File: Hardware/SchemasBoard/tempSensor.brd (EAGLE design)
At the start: 19.4 x 19 mm, 14 parts, among them IC1 DS1820, T1 BC846

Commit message: a
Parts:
- C1: value (none) -> 100nF
- C2: value (none) -> 1uF
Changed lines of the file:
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@@
 <element name="LSP1" library="solpad" package="LSP11" value="LSP11" x="2.54" y="1.3716"/>
 <element name="LSP2" library="solpad" package="LSP11" value="LSP11" x="15.1384" y="1.3208"/>
-<element name="C1" library="resistor" package="C2012" value="" x="12.5603" y="16.3703" rot="MR90"/>
+<element name="C1" library="resistor" package="C2012" value="100nF" x="12.5603" y="16.3703" rot="MR90"/>
 <element name="S1" library="switch-dil" package="SD4-01" value="" x="5.7658" y="5.9436" rot="R90">
 <attribute name="OC_NEWARK" value="unknown" x="5.7658" y="5.9436" size="1.778" layer="27" rot="R90" display="off"/>
@@
 <attribute name="OC_FARNELL" value="unknown" x="5.7658" y="5.9436" size="1.778" layer="27" rot="R90" display="off"/>
 </element>
-<element name="C2" library="resistor" package="SMC_A" value="" x="14.4145" y="15.9893" rot="MR90"/>
+<element name="C2" library="resistor" package="SMC_A" value="1uF" x="14.4145" y="15.9893" rot="MR90"/>
 <element name="R1" library="resistor" package="R1206W" value="4K7" x="1.524" y="14.9098" rot="MR90"/>
 <element name="JP1" library="pinhead" package="1X03" value="" x="15.2781" y="4.5212"/>

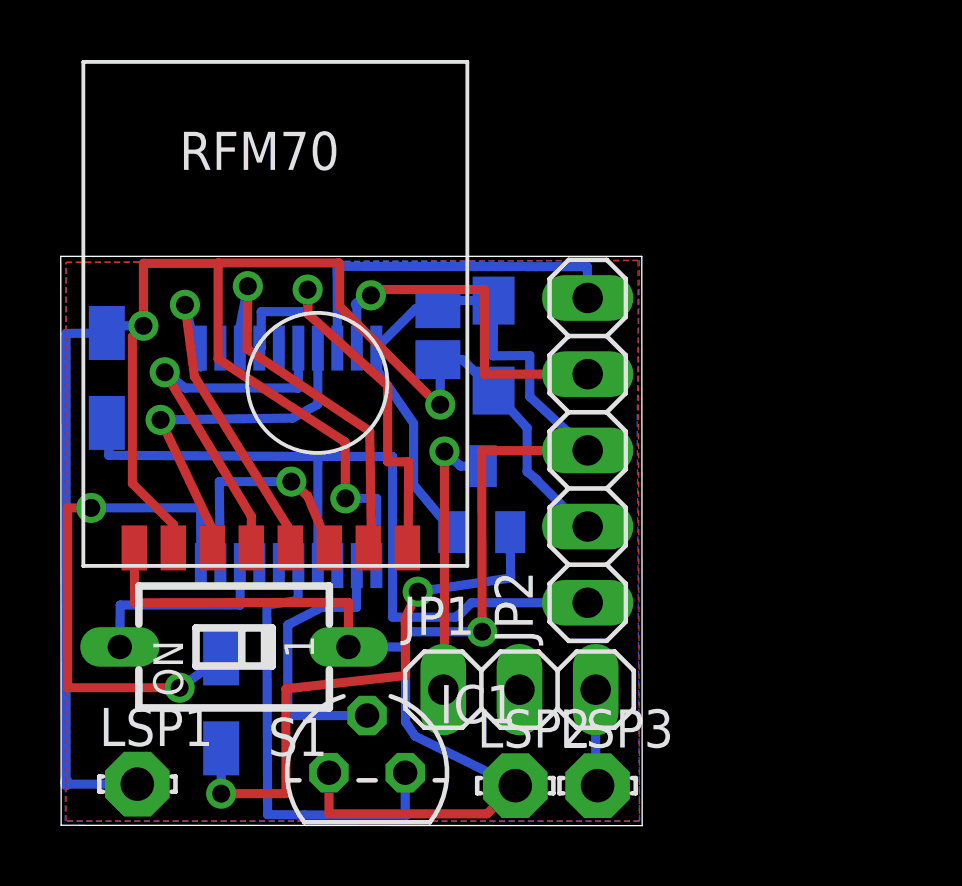
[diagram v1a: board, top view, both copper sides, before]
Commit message: aaa
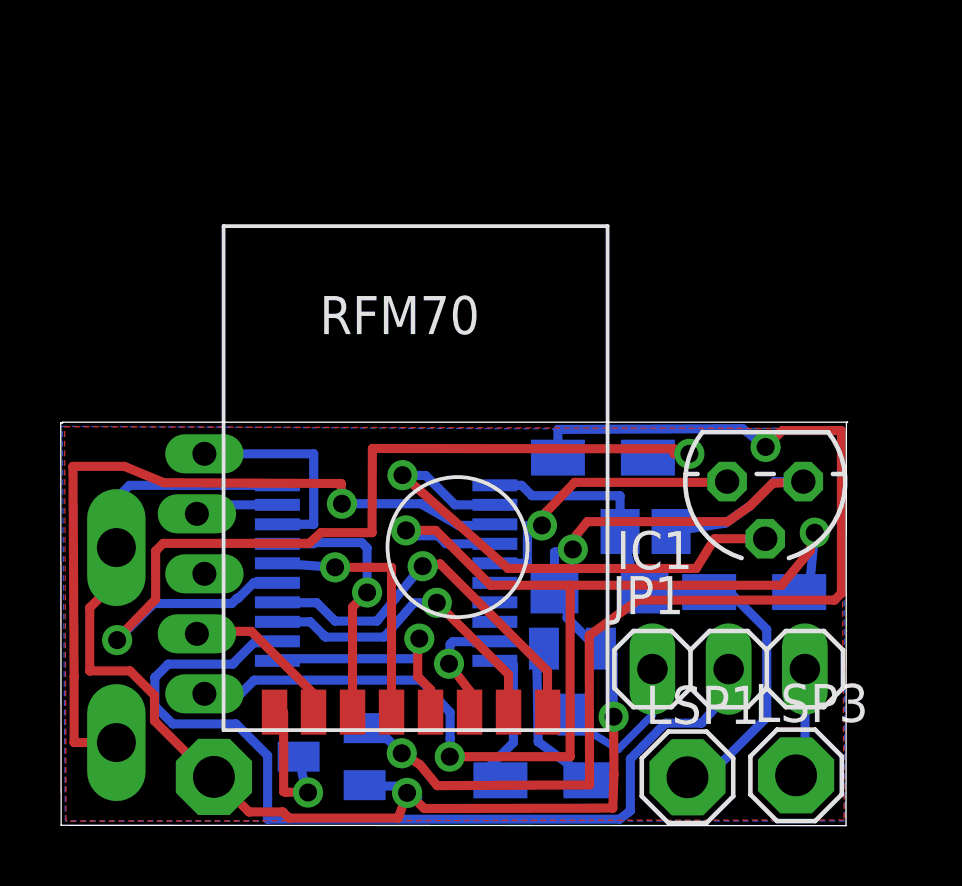
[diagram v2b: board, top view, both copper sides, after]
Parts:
- removed JP2: Prog, pinhead:1X05
- added R3: 1K, resistor:R1206W
- added T2: BC846, transistor:SOT23
- added U$3: PROGRAMMINGHEADERDIP, rfm70:PROGHEADER
- LSP1, LSP2, LSP3: value LSP11 -> SE14; device solpad:LSP11 -> solpad:SE14
- S1: value (none) -> DTS-3; device switch-dil:SD4-01 -> switch-tact:DTS-3
- moved R1 22.7 mm to (23.1, 7.77), turned to 0 degrees
- moved LSP1 18.3 mm to (20.9, 1.60)
- moved IC1 16.4 mm to (23.5, 11.5), turned to 180 degrees
- moved R2 11.1 mm to (16.1, 1.50), turned to 0 degrees
- moved LSP2 10.0 mm to (5.09, 1.61), flipped to the bottom
- moved C1 9.55 mm to (19.5, 9.79), turned to 180 degrees
- moved C2 8.95 mm to (17.9, 7.76), turned to 0 degrees
- moved U$1 7.20 mm to (7.21, 18.1)
- moved JP1 7.01 mm to (22.3, 5.21)
- moved T1 6.79 mm to (17.0, 4.79), turned to 180 degrees
- moved LSP3 6.63 mm to (24.5, 1.66)
- moved U$2 5.06 mm to (10.8, 8.41), turned to 270 degrees
- moved S1 3.92 mm to (1.84, 6.01), flipped to the bottom, turned to 270 degrees
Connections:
- removed net N$18: JP2.4, U$2.19
- removed net N$19: JP2.5, U$2.18
- new net N$10: U$3.GND
- new net N$11: U$2.18, U$3.PGC
- new net N$13: T2.3, U$1.GND
- new net N$14: R3.2, T2.1
- new net N$15: R3.1, U$2.15
- new net N$8: U$2.19, U$3.PGD
- net GND: now also T2.2; no longer JP2.3, U$1.GND
- net N$2: now also U$2.3; no longer U$2.8
- net N$25: now also U$3.MCLR; no longer JP2.1
- net N$4: now also JP1.2
- net VDD: now also U$3.VDD; no longer JP2.2
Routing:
- net VDD: track 66.1 -> 24.1 mm, vias 3 -> 0
- net N$14: track 0.00 -> 38.4 mm, vias 0 -> 2
- net N$15: track 0.00 -> 32.1 mm, vias 0 -> 2
- net N$4: track 0.00 -> 31.0 mm
- net N$2: track 6.71 -> 25.7 mm, vias 0 -> 1
- net N$25: track 26.3 -> 40.8 mm, vias 0 -> 3
- net N$7: track 18.7 -> 5.51 mm, vias 2 -> 0
- net N$6: track 17.8 -> 4.98 mm, vias 2 -> 0
- net N$18: track 12.3 -> 0.00 mm, vias 1 -> 0
- net N$19: track 12.1 -> 0.00 mm
- net N$1: track 9.47 -> 17.3 mm, vias 0 -> 1
- net N$11: track 0.00 -> 7.21 mm
- net N$3: track 15.3 -> 9.75 mm, vias 0 -> 1
- net N$13: track 0.00 -> 5.01 mm, vias 0 -> 1
- net N$23: track 8.44 -> 4.03 mm
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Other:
- board size 19.4 x 19 mm -> 26.2 x 13.4 mm
